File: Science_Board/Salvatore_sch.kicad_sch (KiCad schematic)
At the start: 7 parts, among them U3 PCA9685PW

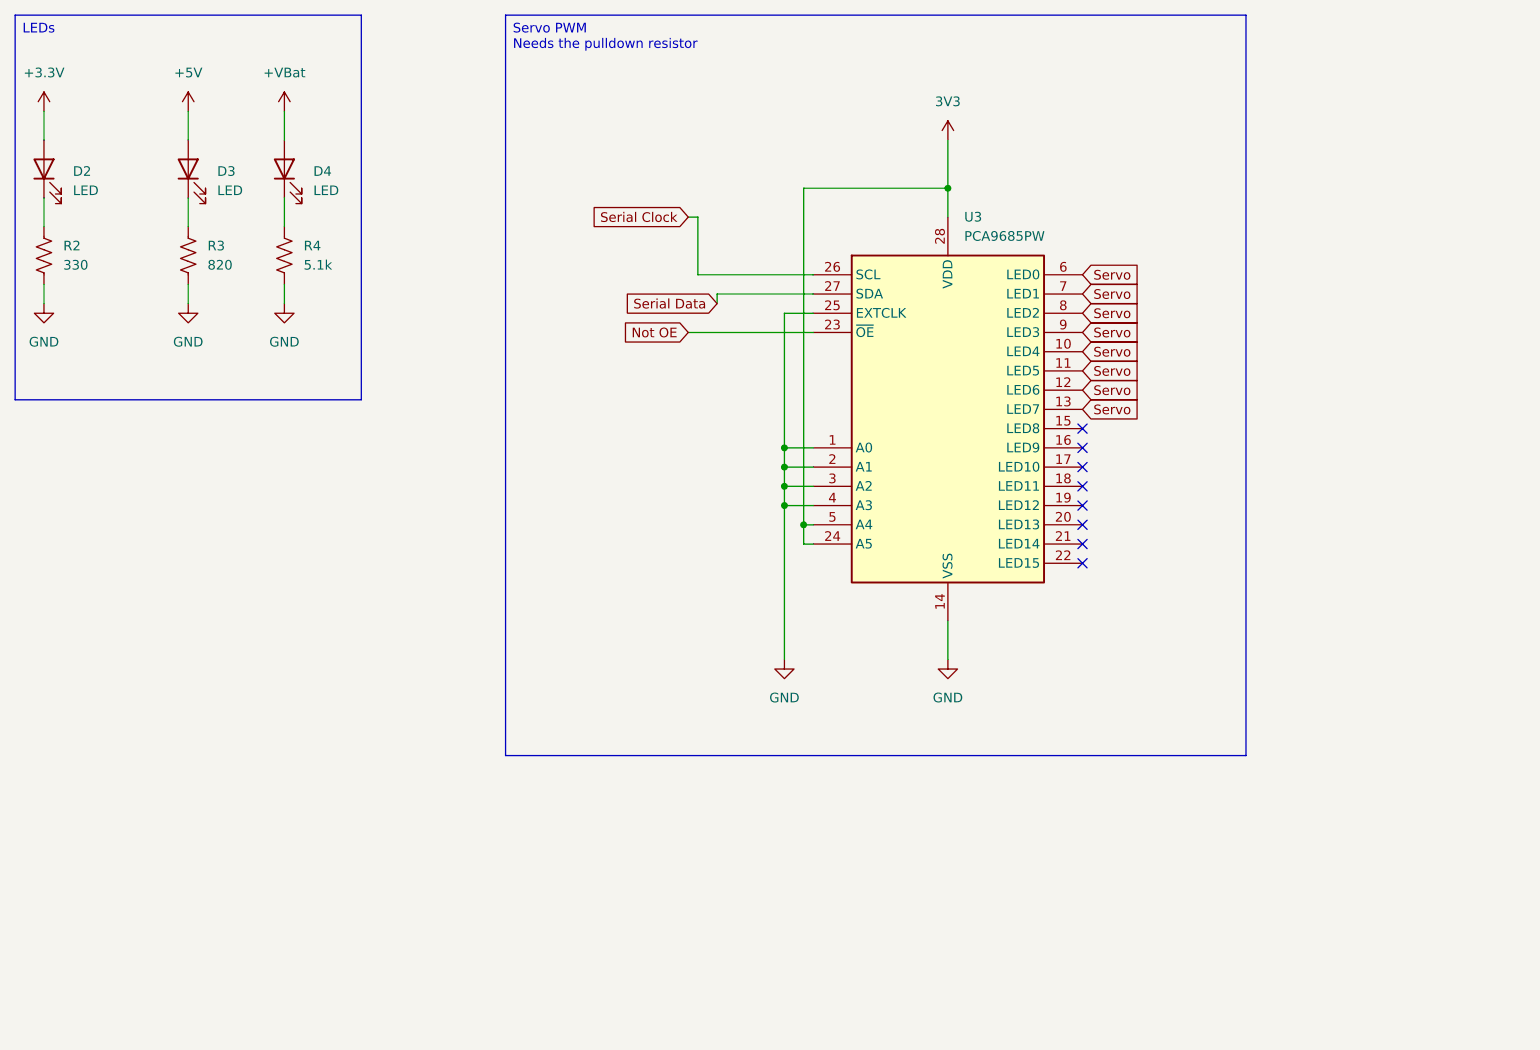
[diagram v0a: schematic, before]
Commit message: EFuses
They done
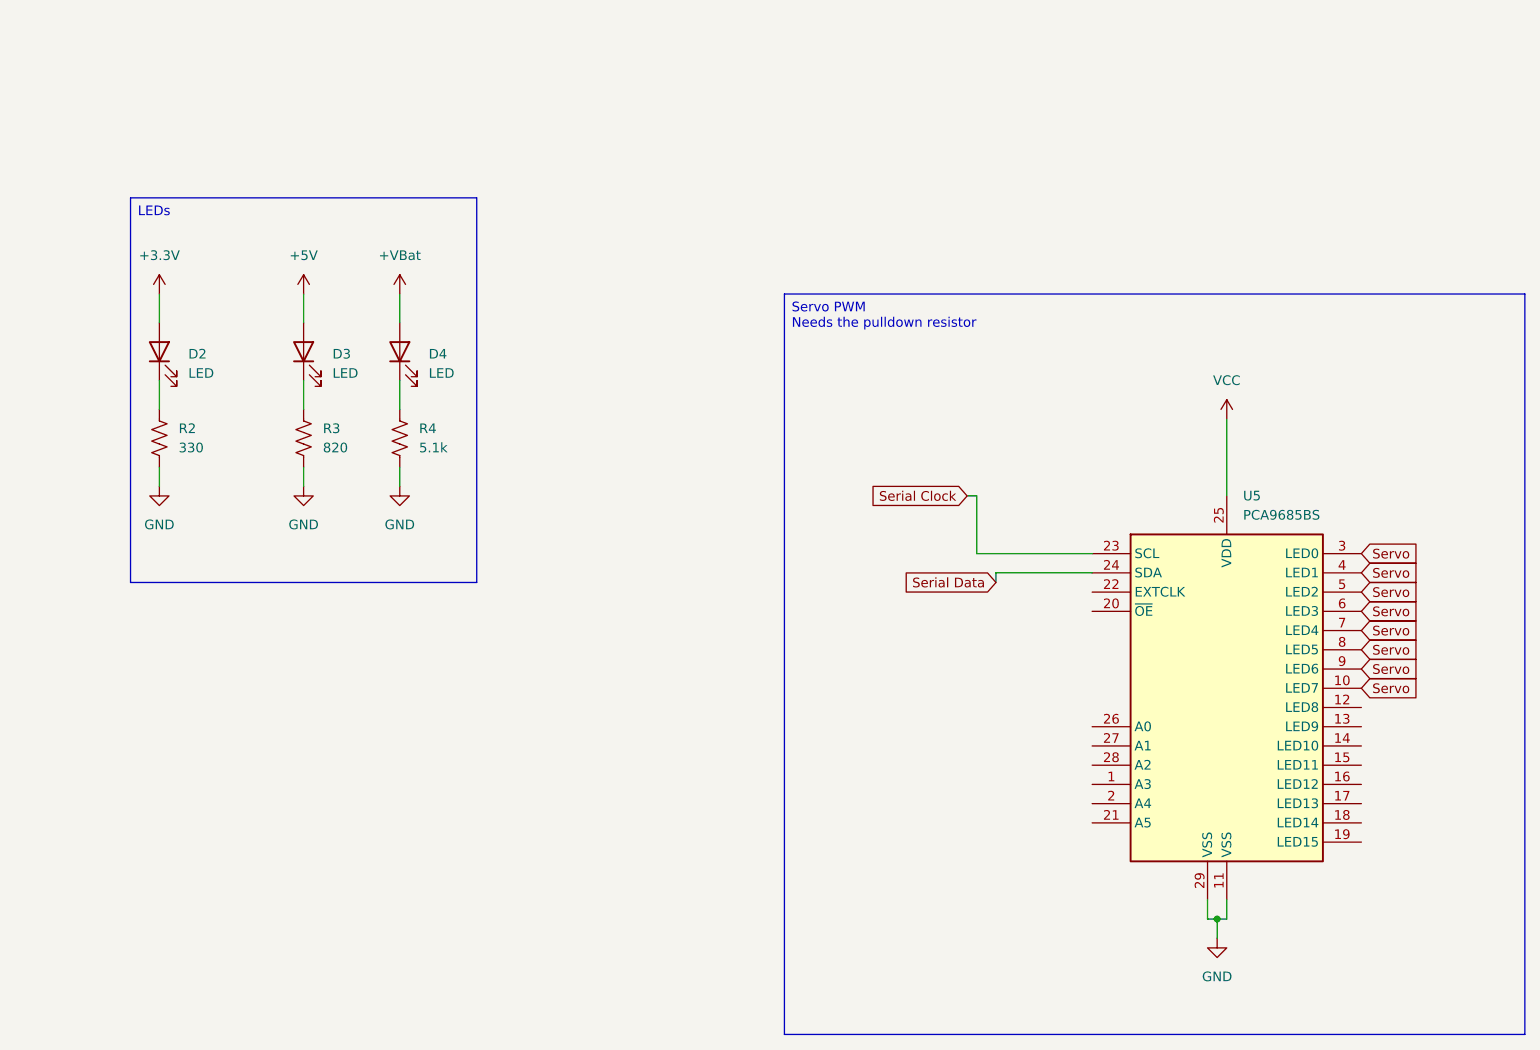
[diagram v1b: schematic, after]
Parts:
- removed U3: PCA9685PW, Package_SO:TSSOP-28_4.4x9.7mm_P0.65mm, symbol Driver_LED:PCA9685PW
- added U5: PCA9685BS, Package_DFN_QFN:QFN-28-1EP_6x6mm_P0.65mm_EP4.25x4.25mm, symbol Driver_LED:PCA9685BS
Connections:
- net GND: now also U5.11 (VSS), U5.29 (VSS)
- net Serial Clock: now also U5.23 (SCL)
- net Serial Data: now also U5.24 (SDA)
- net Servo: now also U5.10 (LED7), U5.3 (LED0), U5.4 (LED1), U5.5 (LED2), U5.6 (LED3), U5.7 (LED4), U5.8 (LED5), U5.9 (LED6)
- new net VCC: U5.25 (VDD)
- no-connect marks 8 -> 0
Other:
- moved on the sheet: D2, D3, D4, R2, R3, R4
